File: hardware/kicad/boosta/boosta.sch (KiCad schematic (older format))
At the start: 2 parts, among them J1 Conn_01x08_Female, J2 Screw_Terminal_01x02

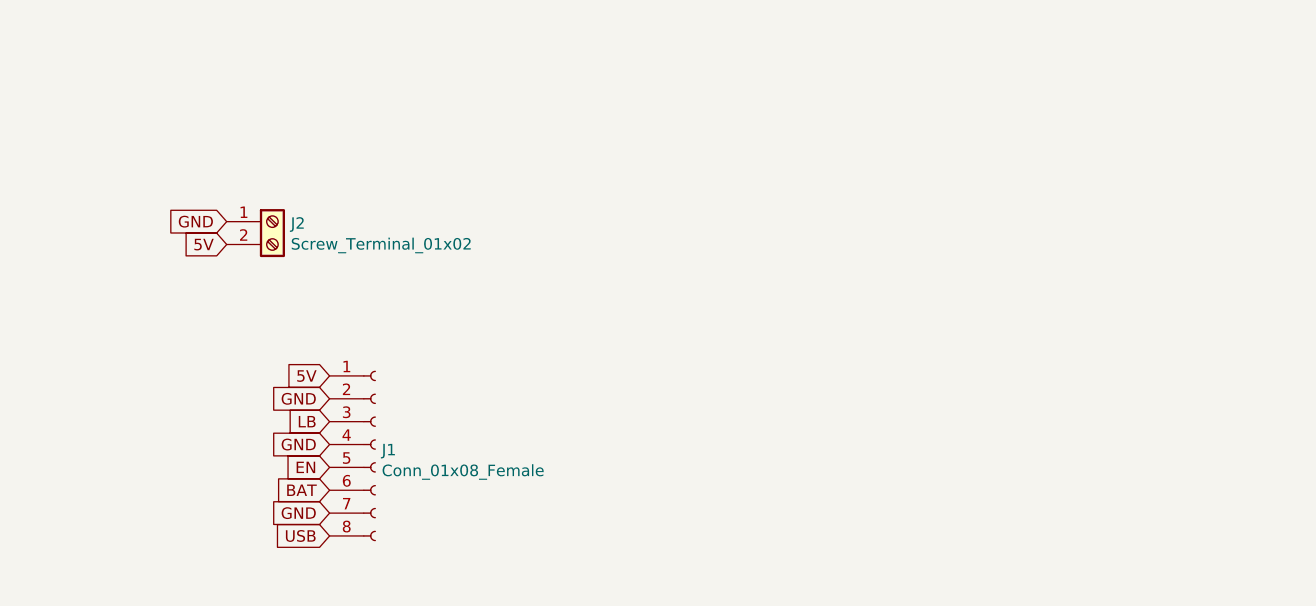
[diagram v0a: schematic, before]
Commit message: update
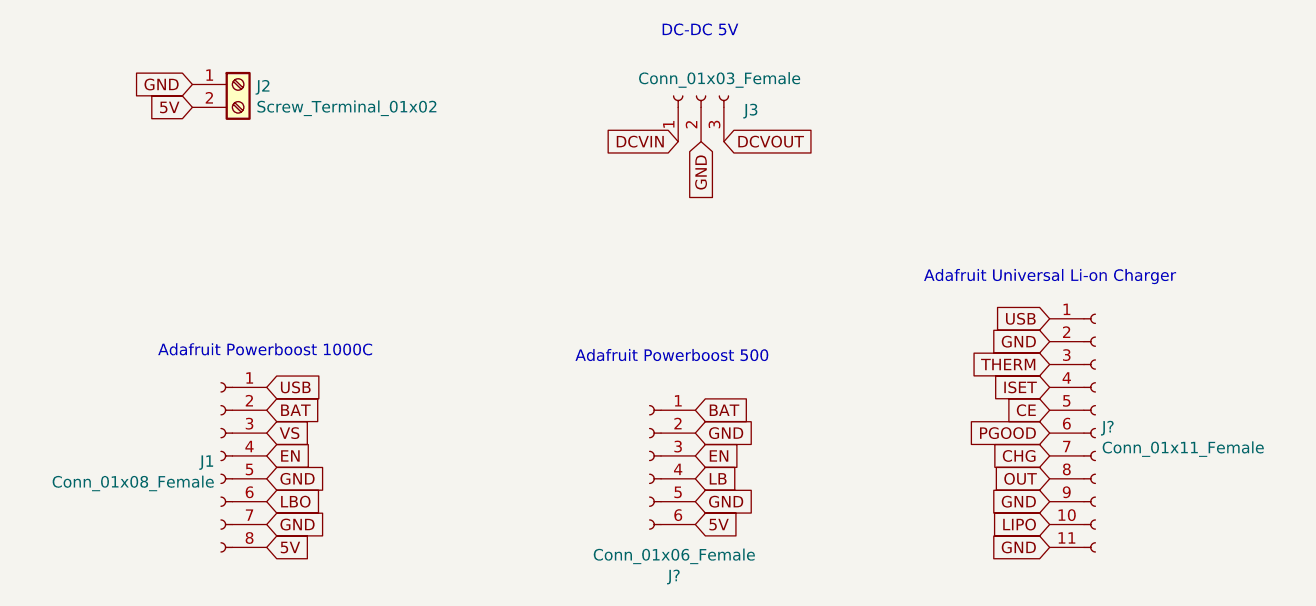
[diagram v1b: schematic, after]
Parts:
- added J3: Conn_01x03_Female, Connector_PinSocket_2.54mm:PinSocket_1x03_P2.54mm_Vertical, symbol Connector:Conn_01x03_Female
- added J?: Conn_01x06_Female, symbol Connector:Conn_01x06_Female
- added J?: Conn_01x11_Female, symbol Connector:Conn_01x11_Female
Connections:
- net 5V: now also J1.8 (Pin_8), J?.6 (Pin_6); no longer J1.1 (Pin_1)
- net BAT: now also J1.2 (Pin_2), J?.1 (Pin_1); no longer J1.6 (Pin_6)
- net EN: now also J1.4 (Pin_4), J?.3 (Pin_3); no longer J1.5 (Pin_5)
- net GND: now also J1.5 (Pin_5), J3.2 (Pin_2), J?.11 (Pin_11), J?.2 (Pin_2), J?.2 (Pin_2), J?.5 (Pin_5), J?.9 (Pin_9); no longer J1.2 (Pin_2), J1.4 (Pin_4)
- net LB: now also J?.4 (Pin_4); no longer J1.3 (Pin_3)
- net USB: now also J1.1 (Pin_1), J?.1 (Pin_1); no longer J1.8 (Pin_8)
- new net CE: J?.5 (Pin_5)
- new net CHG: J?.7 (Pin_7)
- new net DCVIN: J3.1 (Pin_1)
- new net DCVOUT: J3.3 (Pin_3)
- new net ISET: J?.4 (Pin_4)
- new net LBO: J1.6 (Pin_6)
- new net LIPO: J?.10 (Pin_10)
- new net OUT: J?.8 (Pin_8)
- new net PGOOD: J?.6 (Pin_6)
- new net THERM: J?.3 (Pin_3)
- new net VS: J1.3 (Pin_3)
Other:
- note added: "Adafruit Powerboost 1000C"
- note added: "Adafruit Powerboost 500"
- note added: "Adafruit Universal Li-on Charger"
- note added: "DC-DC 5V"
- moved on the sheet: J1, J2
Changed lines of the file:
@@
 L Connector:Conn_01x08_Female J1
 U 1 1 612E5F14
-P 2100 2675
-F 0 "J1" H 2128 2651 50  0000 L CNN
-F 1 "Conn_01x08_Female" H 2128 2560 50  0000 L CNN
-F 2 "Connector_PinSocket_2.54mm:PinSocket_1x08_P2.54mm_Vertical" H 2100 2675 50  0001 C CNN
-F 3 "~" H 2100 2675 50  0001 C CNN
-	1    2100 2675
-	1    0    0    -1
+P 1425 2725
+F 0 "J1" H 1453 2701 50  0000 L CNN
+F 1 "Conn_01x08_Female" H 1453 2610 50  0000 L CNN
+F 2 "Connector_PinSocket_2.54mm:PinSocket_1x08_P2.54mm_Vertical" H 1425 2725 50  0001 C CNN
+F 3 "~" H 1425 2725 50  0001 C CNN
+	1    1425 2725
+	-1   0    0    -1
 $EndComp
-Text GLabel 1900 2375 0    50   Input ~ 0
+Text GLabel 1625 3125 2    50   Input ~ 0
 5V
-Text GLabel 1900 2475 0    50   Input ~ 0
+Text GLabel 1625 3025 2    50   Input ~ 0
 GND
-Text GLabel 1900 2575 0    50   Input ~ 0
-LB
-Text GLabel 1900 2675 0    50   Input ~ 0
+Text GLabel 1625 2925 2    50   Input ~ 0
+LBO
+Text GLabel 1625 2825 2    50   Input ~ 0
 GND
-Text GLabel 1900 2775 0    50   Input ~ 0
-EN
-Text GLabel 1900 2875 0    50   Input ~ 0
+Text GLabel 1625 2625 2    50   Input ~ 0
+VS
+Text GLabel 1625 2525 2    50   Input ~ 0
 BAT
-Text GLabel 1900 2975 0    50   Input ~ 0
-GND
-Text GLabel 1900 3075 0    50   Input ~ 0
+Text GLabel 1625 2425 2    50   Input ~ 0
 USB
 $Comp
 L Connector:Screw_Terminal_01x02 J2
 U 1 1 612EBB78
-P 1650 1700
-F 0 "J2" H 1730 1692 50  0000 L CNN
-F 1 "Screw_Terminal_01x02" H 1730 1601 50  0000 L CNN
-F 2 "TerminalBlock_Phoenix:TerminalBlock_Phoenix_MKDS-1,5-2-5.08_1x02_P5.08mm_Horizontal" H 1650 1700 50  0001 C CNN
-F 3 "~" H 1650 1700 50  0001 C CNN
-	1    1650 1700
+P 1500 1100
+F 0 "J2" H 1580 1092 50  0000 L CNN
+F 1 "Screw_Terminal_01x02" H 1580 1001 50  0000 L CNN
+F 2 "TerminalBlock_Phoenix:TerminalBlock_Phoenix_MKDS-1,5-2-5.08_1x02_P5.08mm_Horizontal" H 1500 1100 50  0001 C CNN
+F 3 "~" H 1500 1100 50  0001 C CNN
+	1    1500 1100
 	1    0    0    -1
 $EndComp
-Text GLabel 1450 1700 0    50   Input ~ 0
+Text GLabel 1300 1100 0    50   Input ~ 0
 GND
-Text GLabel 1450 1800 0    50   Input ~ 0
+Text GLabel 1300 1200 0    50   Input ~ 0
 5V
+$Comp
+L Connector:Conn_01x03_Female J3
+U 1 1 612FD2B7
+P 3525 1150
+F 0 "J3" V 3463 962 50  0000 R CNN
+F 1 "Conn_01x03_Female" V 3600 1425 50  0000 R CNN
+F 2 "Connector_PinSocket_2.54mm:PinSocket_1x03_P2.54mm_Vertical" H 3525 1150 50  0001 C CNN
+F 3 "~" H 3525 1150 50  0001 C CNN
+	1    3525 1150
+	0    -1   -1   0
+$EndComp
+Text GLabel 3425 1350 0    50   Input ~ 0
+DCVIN
+Text GLabel 3525 1350 3    50   Input ~ 0
+GND
+Text GLabel 3625 1350 2    50   Input ~ 0
+DCVOUT
+$Comp
+L Connector:Conn_01x06_Female J?
+U 1 1 61547B30
+P 3300 2725
+F 0 "J?" H 3192 2200 50  0000 C CNN
+F 1 "Conn_01x06_Female" H 3192 2291 50  0000 C CNN
+F 2 "" H 3300 2725 50  0001 C CNN
+F 3 "~" H 3300 2725 50  0001 C CNN
+	1    3300 2725
+	-1   0    0    -1
+$EndComp
+Text GLabel 3500 3025 2    50   Input ~ 0
+5V
+Text GLabel 3500 2925 2    50   Input ~ 0
+GND
+Text GLabel 3500 2825 2    50   Input ~ 0
+LB
+Text GLabel 3500 2725 2    50   Input ~ 0
+EN
+Text GLabel 3500 2625 2    50   Input ~ 0
+GND
+Text GLabel 3500 2525 2    50   Input ~ 0
+BAT
+Text GLabel 1625 2725 2    50   Input ~ 0
+EN
+Text Notes 1150 2300 0    50   ~ 0
+Adafruit Powerboost 1000C
+Text Notes 2975 2325 0    50   ~ 0
+Adafruit Powerboost 500
+Text Notes 3350 900  0    50   ~ 0
+DC-DC 5V
+Text Notes 4500 1975 0    50   ~ 0
+Adafruit Universal Li-on Charger
+$Comp
+L Connector:Conn_01x11_Female J?
+U 1 1 6155BE06
+P 5250 2625
+F 0 "J?" H 5278 2651 50  0000 L CNN
+F 1 "Conn_01x11_Female" H 5278 2560 50  0000 L CNN
+F 2 "" H 5250 2625 50  0001 C CNN
+F 3 "~" H 5250 2625 50  0001 C CNN
+	1    5250 2625
+	1    0    0    -1
+$EndComp
+Text GLabel 5050 2125 0    50   Input ~ 0
+USB
+Text GLabel 5050 2225 0    50   Input ~ 0
+GND
+Text GLabel 5050 2325 0    50   Input ~ 0
+THERM
+Text GLabel 5050 2425 0    50   Input ~ 0
+ISET
+Text GLabel 5050 2525 0    50   Input ~ 0
+CE
+Text GLabel 5050 2625 0    50   Input ~ 0
+PGOOD
+Text GLabel 5050 2725 0    50   Input ~ 0
+CHG
+Text GLabel 5050 2825 0    50   Input ~ 0
+OUT
+Text GLabel 5050 2925 0    50   Input ~ 0
+GND
+Text GLabel 5050 3025 0    50   Input ~ 0
+LIPO
+Text GLabel 5050 3125 0    50   Input ~ 0
+GND
 $EndSCHEMATC
